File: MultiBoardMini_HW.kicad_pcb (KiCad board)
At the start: 2 copper layers, 63 x 63 mm, 56 parts, among them J1 PB0, J2 PA10, J3 Conn_01x02_Male, J4 PA10, J6 Conn_01x04, SW1 PF1, SW2 RESET, SW3 SW_Push_DPDT, SW5 SW_Push_DPDT, T3 PTS_1.5_2, U1 M78AR5-1, U2 NUCLEO-F303K8, U3 ESP32-C3-WROOM-02-N4, U4 TB67H303HG, U5 TB67H303HG, U6 MCP2562-E_SN

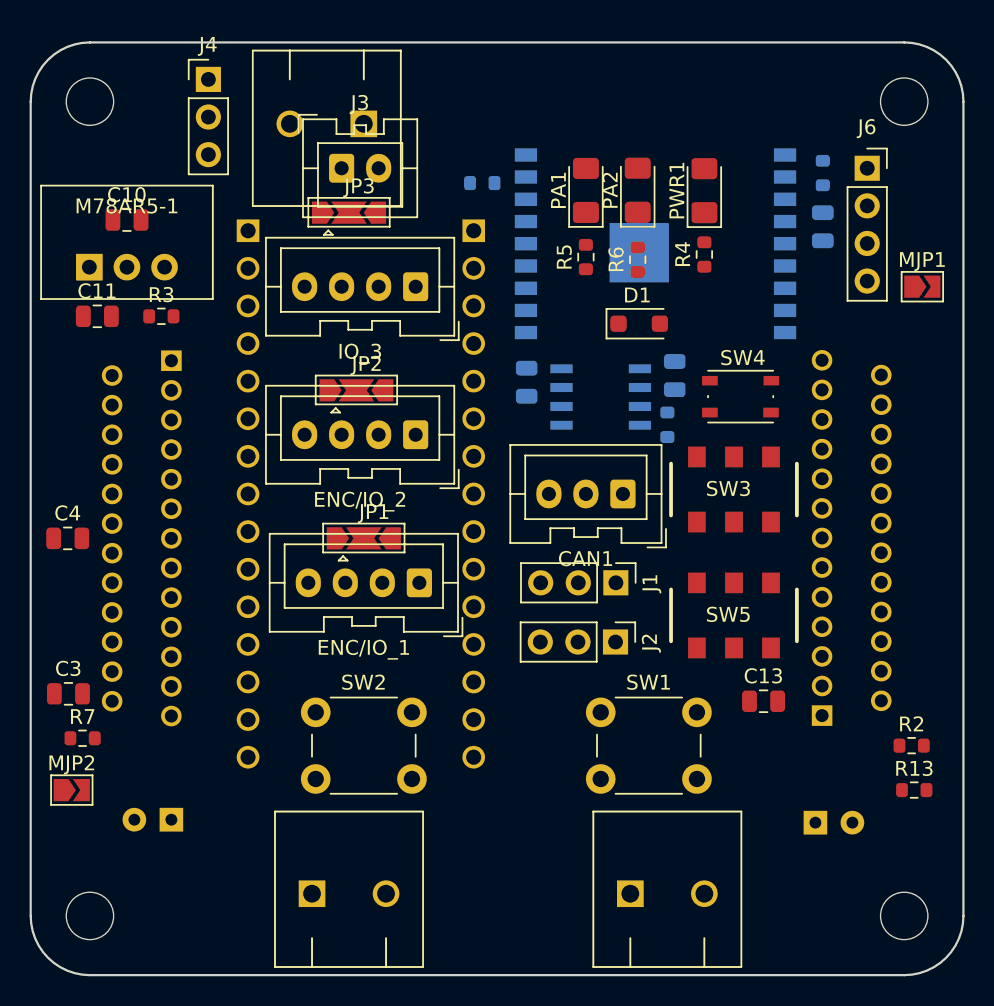
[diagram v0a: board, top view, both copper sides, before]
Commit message: 部品は一おおむね完了
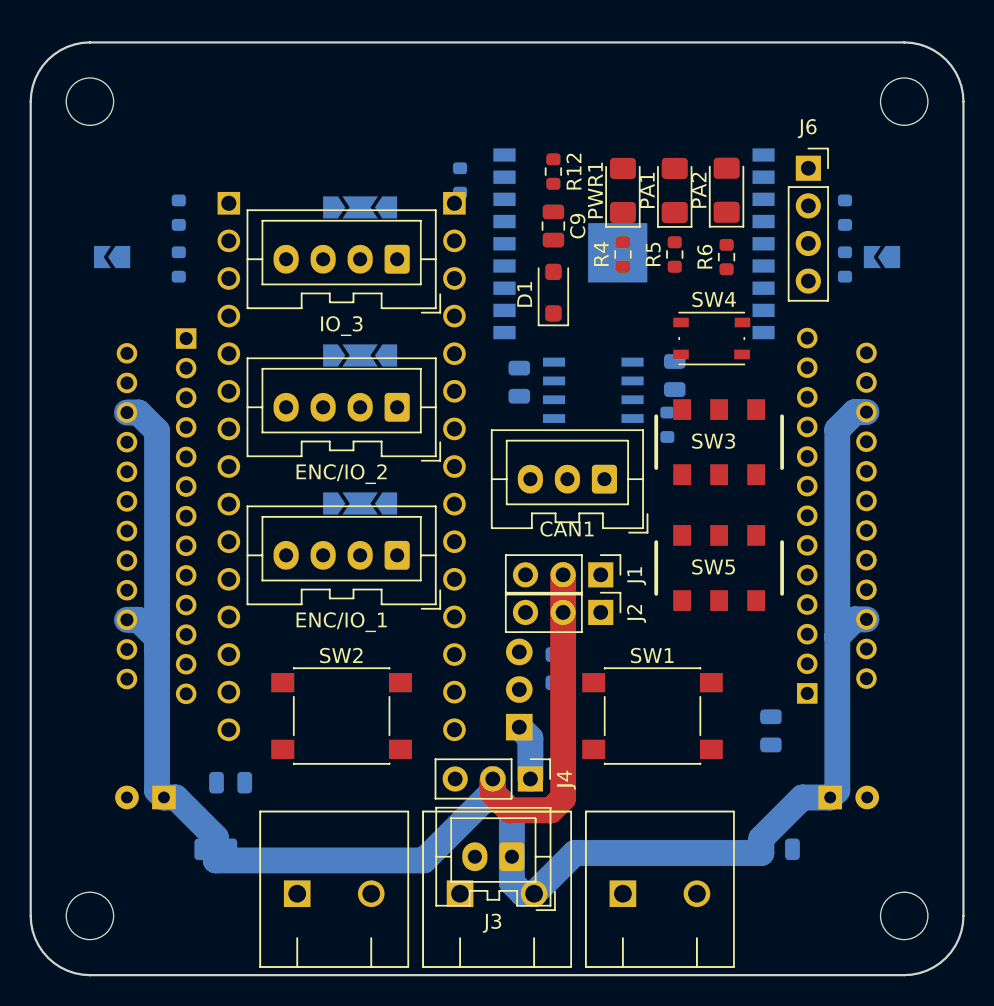
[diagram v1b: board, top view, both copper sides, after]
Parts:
- removed ? (x4): , 
- added REF3: MountingHole_3.2mm_M3, MountingHole:MountingHole_3.2mm_M3, F.Cu at (27.5, -27.5)
- added REF3: MountingHole_3.2mm_M3, MountingHole:MountingHole_3.2mm_M3, F.Cu at (-27.5, -27.5)
- added REF3: MountingHole_3.2mm_M3, MountingHole:MountingHole_3.2mm_M3, F.Cu at (-27.5, 27.5)
- added REF3: MountingHole_3.2mm_M3, MountingHole:MountingHole_3.2mm_M3, F.Cu at (27.5, 27.5)
- C10, C11, C13, C3, C4, JP1, JP2, JP3, MJP1, MJP2, R13, R2, R3, R7, U1: moved to B.Cu
- C9, R12: moved to F.Cu
- SW1, SW2: footprint Button_Switch_THT:SW_PUSH_6mm_H4.3mm -> Button_Switch_SMD:SW_Push_1P1T_NO_6x6mm_H9.5mm
- moved C11 58.4 mm to (19.0, 23.0)
- moved T3 53.3 mm to (0.00, 26.0), turned to 0 degrees
- moved J4 52.0 mm to (2.25, 18.2), turned to -90 degrees
- moved J3 47.9 mm to (1.00, 23.5), turned to 180 degrees
- moved C10 41.9 mm to (4.00, 10.8), turned to -90 degrees
- moved R13 39.3 mm to (23.5, -20.0), turned to 90 degrees
- moved U1 38.9 mm to (1.50, 12.2), turned to 90 degrees
- moved MJP2 36.1 mm to (-26.0, -17.0), turned to 180 degrees
- moved R7 36.1 mm to (-21.5, -20.0), turned to 90 degrees
- moved R2 32.8 mm to (23.5, -16.5), turned to 90 degrees
- moved C4 23.3 mm to (-19.0, 23.0), turned to 180 degrees
- moved R12 18.2 mm to (3.81, -22.8)
- moved C9 18.2 mm to (3.81, -19.1)
- moved C3 12.5 mm to (-18.0, 18.5)
- moved D1 6.16 mm to (3.81, -14.6), turned to 90 degrees
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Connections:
- CAN1 pad 2: unconnected-(CAN1-Pin_2-Pad2) -> Net-(CAN1-Pin_2)
- CAN1 pad 3: unconnected-(CAN1-Pin_3-Pad3) -> Net-(CAN1-Pin_3)
- J1 pad 1: GND -> GNDPWR
- J2 pad 1: GND -> GNDPWR
- R1 pad 1: Net-(U6-CANL) -> Net-(CAN1-Pin_2)
- R1 pad 2: Net-(U6-CANH) -> Net-(CAN1-Pin_3)
- U3 pad 9: (no net) -> GND
- U6 pad 6: Net-(U6-CANL) -> Net-(CAN1-Pin_2)
- U6 pad 7: Net-(U6-CANH) -> Net-(CAN1-Pin_3)
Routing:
- net PWR: track 0.00 -> 142.6 mm
- net Net-(J4-Pin_1): track 0.00 -> 3.81 mm
